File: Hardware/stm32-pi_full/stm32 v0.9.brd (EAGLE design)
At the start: 131.4 x 105.8 mm, 278 parts, among them J1 SOLDERJUMPERNO, Q1 MMBT3906, Q2 MMBT3904, Q3 MMBT3904, U1 ESP32-WROOM-32D, Y1 6MM_3.5MM_CRYSTAL

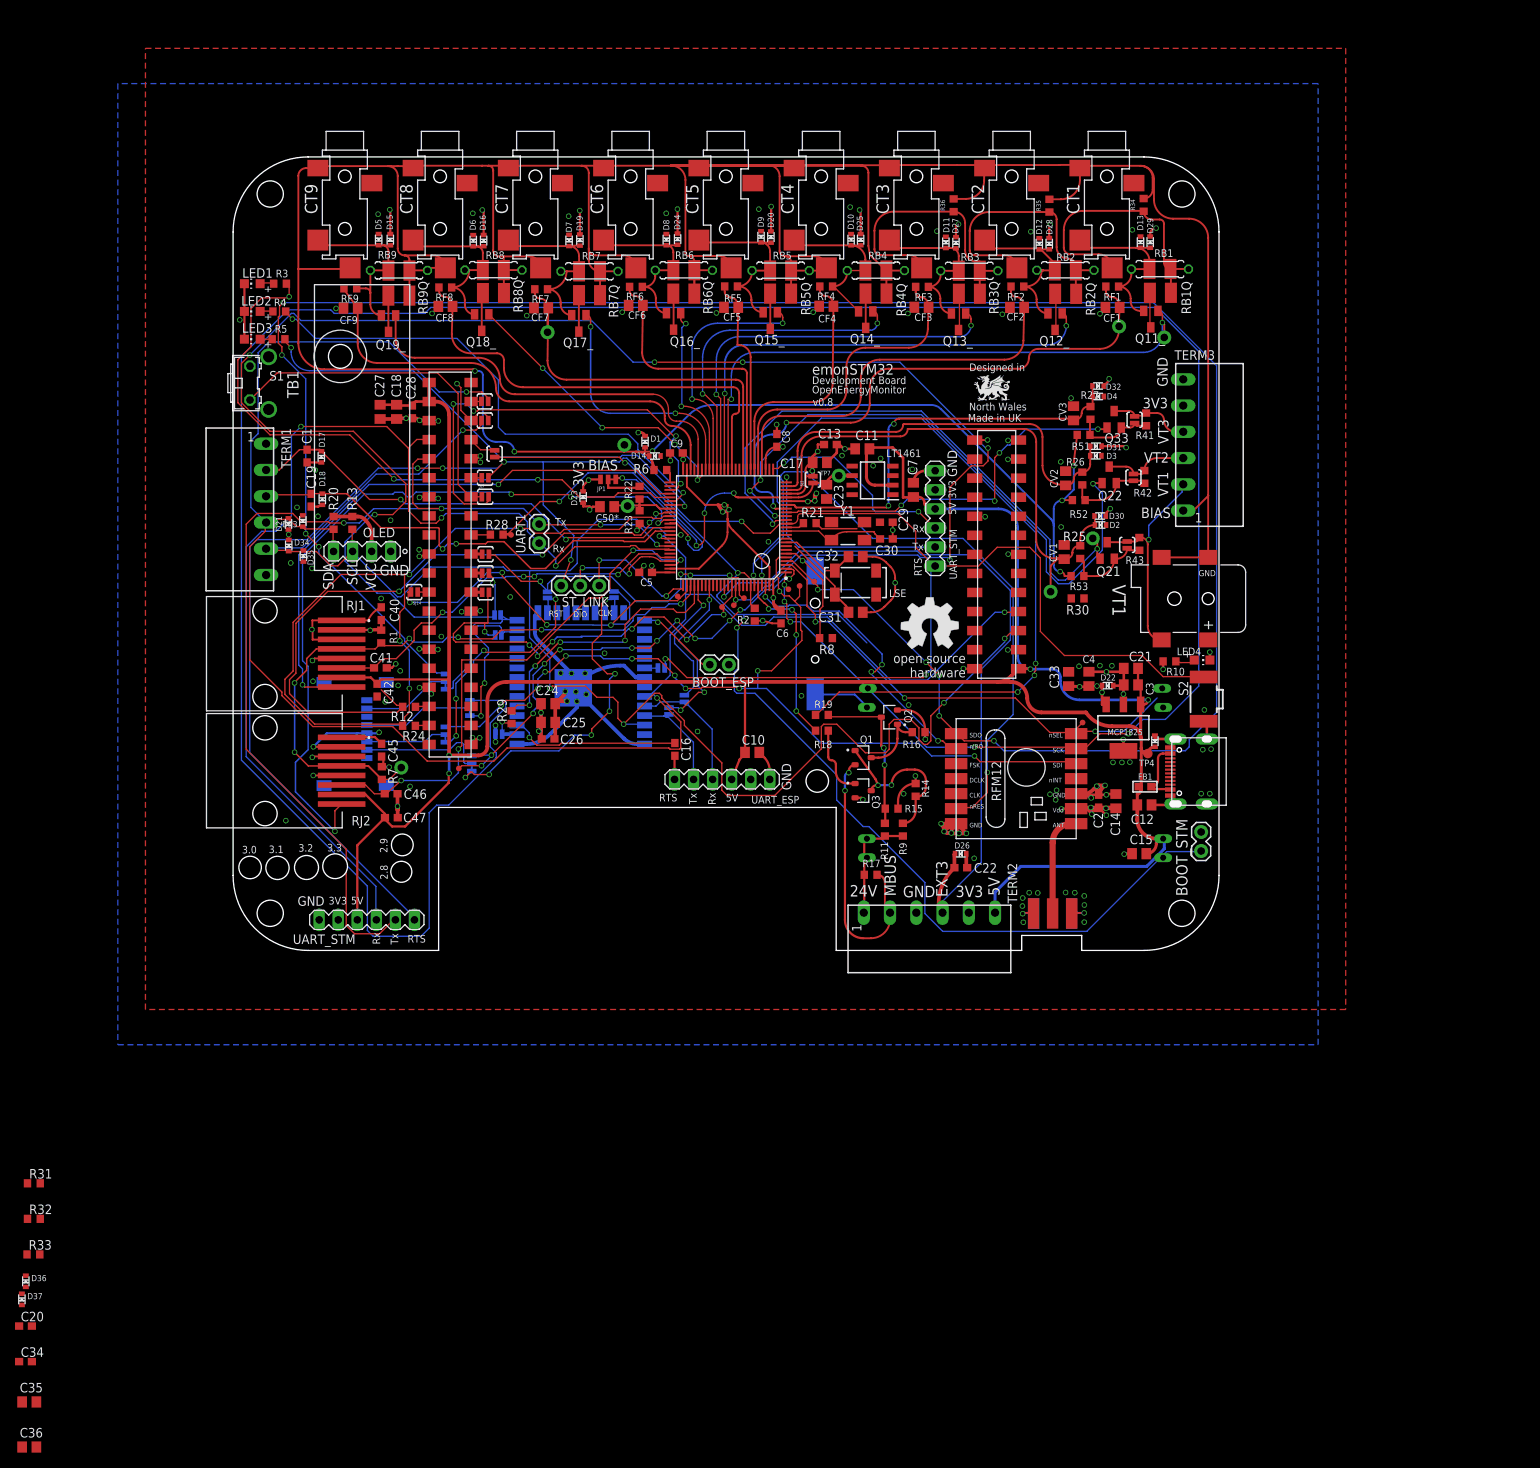
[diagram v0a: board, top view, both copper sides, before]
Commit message: v0.9 backup
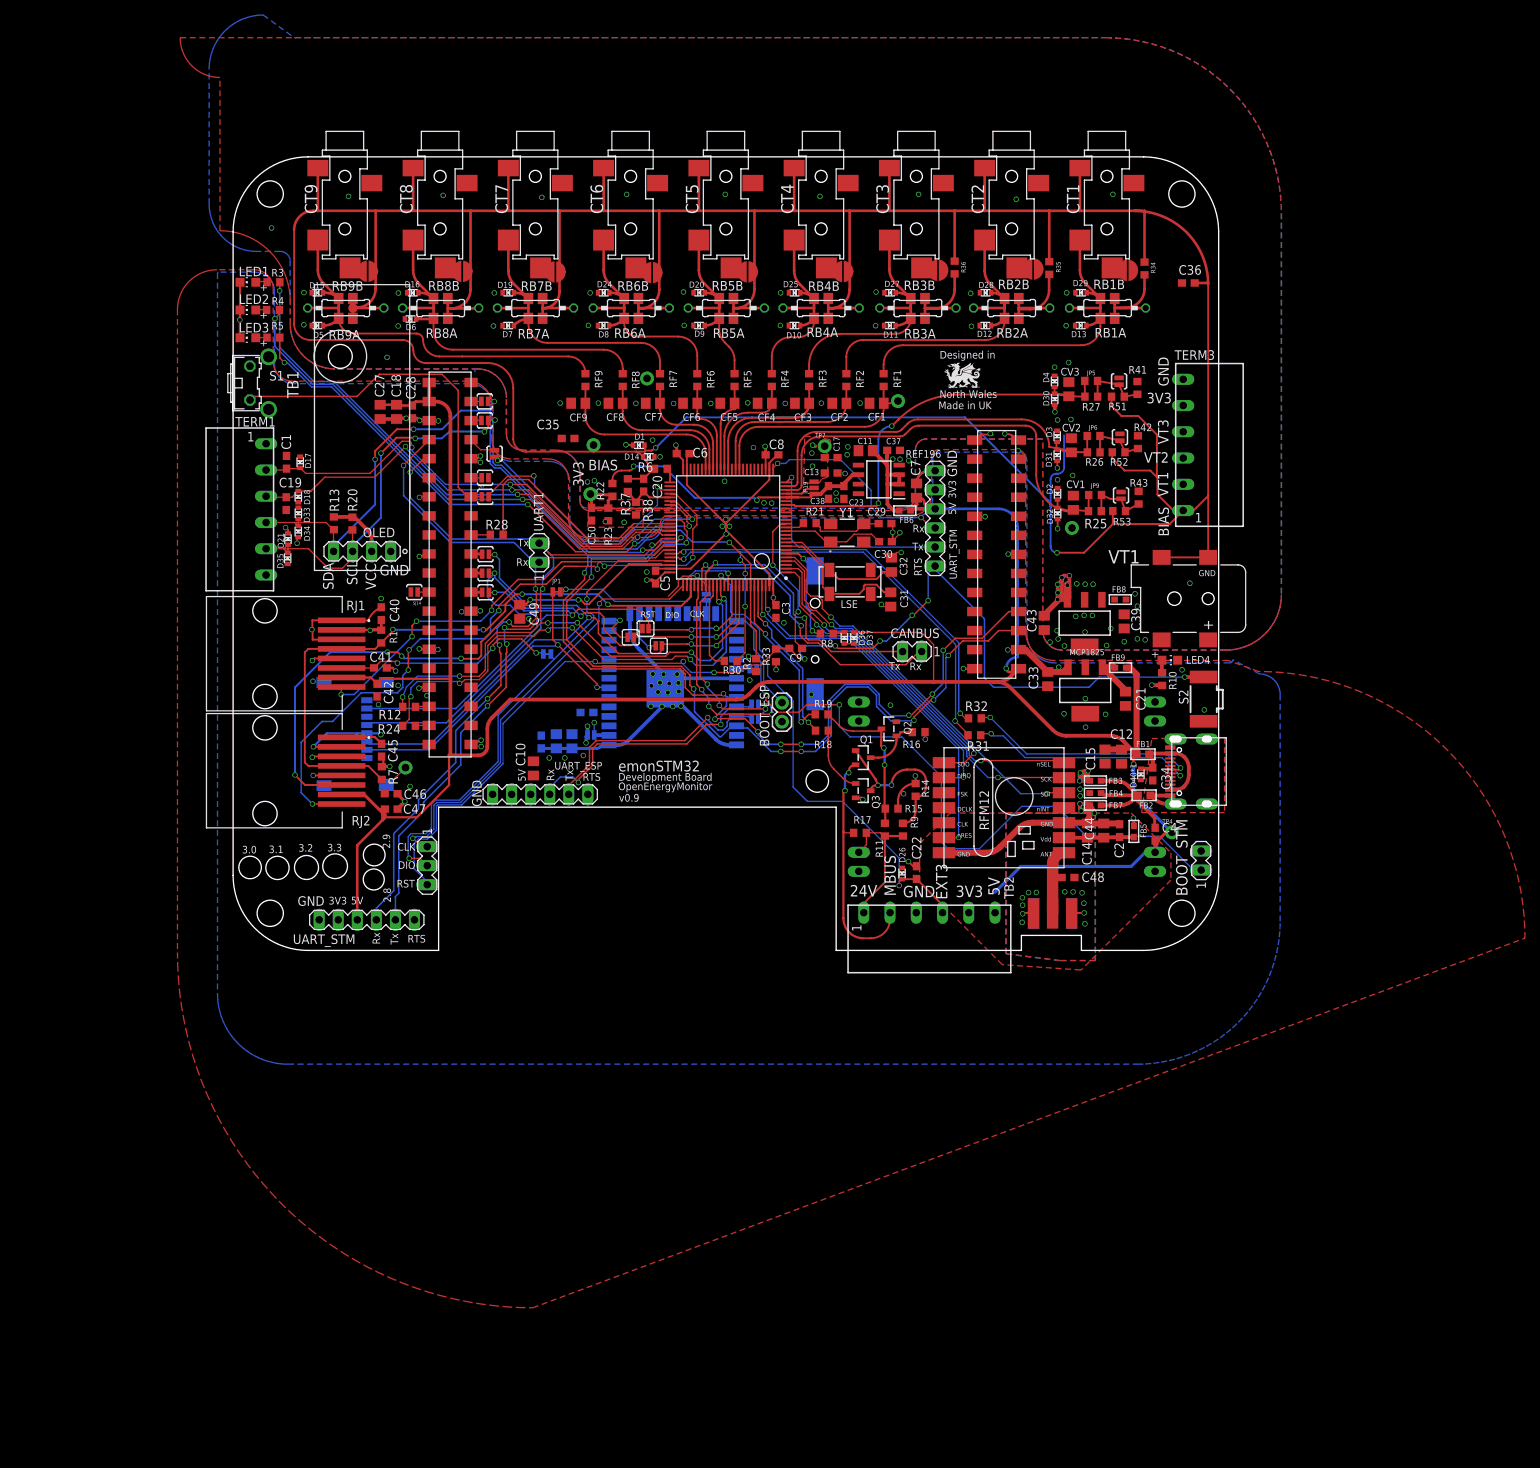
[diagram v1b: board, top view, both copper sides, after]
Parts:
- removed C50*: 2.2uF, rcl:C0805
- removed D22, D23: ESD5Z3.3T1G, microbuilder:SOD-523
- removed GOLD_ORB_SM1: OSHWLOGOLOGO8MM, oshw:OSHW_8MM
- removed JP2, JP3, JP7, JP8: JUMPER-SMT_3_1-NC_TRACE_SILK, SparkFun-Jumpers:SMT-JUMPER_3_1-NC_TRACE_SILK
- removed Q11_, Q12_, Q13_, Q14_, Q15_, Q16_, Q17_, Q18_, Q19_, Q21, Q22, Q33: (no value), adafruit:SOT23
- removed R29: 10K, rcl:R0603
- removed RB1: 22r 0.3W 1%, rcl:R1210
- removed RB1Q, RB2, RB2Q, RB3, RB3Q, RB4, RB4Q, RB5, RB5Q, RB6, RB6Q, RB7, RB7Q, RB8, RB8Q: 22r, rcl:R1210
- removed RB9: 100R 0.1%, rcl:R1210
- removed RB9Q: 22R 0.1%, rcl:R1210
- removed SJ2: SOLDERJUMPERNO, SparkFun:SJ_2S-NO
- removed ST_LINK: 455-1750-1-ND, SparkFun-Connectors:1X03
- removed TP1, TP11, TP12, TP13, TP14, TP15, TP16, TP2, TP21, TP3: TEST-POINT3, SparkFun-Connectors:PAD.03X.03
- removed TP17, TP6: TEST-POINTPOGO_PTH, SparkFun-Connectors:1X01_NO_SILK
- added C37, C38, C48: 100nF, resistor:C0603
- added C39, C43, C44: 22uF, rcl:C0805
- added C49: 10pF, rcl:C0805
- added C50: (no value), rcl:C0603
- added CANBUS: TX/RX, con-lstb-db:MA02-1
- added FB2: (no value), microbuilder:0603
- added FB3, FB4, FB5, FB6, FB7, FB8, FB9: (no value), microbuilder:_0603
- added JP10, JP11, JP12, JP13, JP14, JP15, JP16, JP17, JP18: JUMPER-SMT_2_NO_NO-SILK_ROUND, SparkFun-Jumpers:SMT-JUMPER_2_NO_NO-SILK_ROUND
- added JP19: JUMPER-SMT_3_NO_NO-SILK, SparkFun-Jumpers:SMT-JUMPER_3_NO_NO-SILK
- added JP4: JUMPER-SMT_2_NC_TRACE_NO-SILK, SparkFun-Jumpers:SMT-JUMPER_2_NC_TRACE_NO-SILK
- added JP5, JP6, JP9: 0R, rcl:R0603
- added MCP1825(ANALOG): MCP1825SOT-223-3, SteelCaveRobotics-Power:SOT-223
- added R37: 0R, resistor:R0603
- added R38: 1k, resistor:R0603
- added RB1A, RB1B: 22r 0.3W 1%, rcl:R0805
- added RB2A, RB2B, RB3A, RB3B, RB4A, RB4B, RB5A, RB5B, RB6A, RB6B, RB7A, RB7B, RB8A, RB8B: 22r, rcl:R0805
- added RB9A, RB9B: 100R 0.1%, rcl:R0805
- added SV3: (no value), con-lstb-db:MA03-1
- BOOT_STM, UART1: device SparkFun:1X02 -> con-lstb-db:MA02-1
- C11, C14, C18: value 2.2uF -> 22uF
- C12, C21, C33: value 47uF -> 22uF
- C13, C20: value 100nF -> 2.2uF
- C17, C3, C4: value 2.2uF -> 100nF; device rcl:C0805 -> resistor:C0603
- C23: value 2.2uF -> 1uf; device rcl:C0805 -> rcl:C0603
- C34: device rcl:C0603 -> resistor:C0603
- C35, C36: value 2.2uF -> 1uF; device rcl:C0805 -> rcl:C0603
- C9: value 100nF -> 1uF; device resistor:C0603 -> rcl:C0603
- CT1, CT2, CT3, CT4, CT5, CT6, CT7, CT8, CT9: device IotaWatt_parts:STEREO_SMT -> sj-3523-smt:SJ-352X-SMT
- JP1: value JUMPER-SMT_3_1-NC_TRACE_NO-SILK -> JUMPER-SMT_2_NC_TRACE_NO-SILK; device SparkFun-Jumpers:SMT-JUMPER_3_1-NC_TRACE_NO-SILK -> SparkFun-Jumpers:SMT-JUMPER_2_NC_TRACE_NO-SILK
- Q1: value MMBT3906 -> (none); device Transistor:SOT23 -> microbuilder:SOT23-R
- Q2, Q3: value MMBT3904 -> (none); device Transistor:SOT23 -> microbuilder:SOT23-R
- R25, R26, R27: value 10k -> 9k1
- R30: value 0R -> 1k5; device resistor:R0603 -> rcl:R0603
- R31, R32: value 0R -> 20R; device resistor:R0603 -> rcl:R0603
- R33: value 0R -> 10k
- R41, R42, R43: value 120k -> 100k
- RB1_, RB2_, RB3_, RB4_, RB5_, RB6_, RB7_, RB8_, RB9_: device rcl:0207/7 -> rcl:0207/10
- TP4: value TPB1,27 -> TEST-POINTPOGO_PTH; device testpad:B1,27 -> SparkFun-Connectors:1X01_NO_SILK
- moved C36 219.0 mm to (127.4, 89.0), turned to 180 degrees
- moved C34 169.5 mm to (122.6, 23.5), turned to 270 degrees
- moved C35 147.2 mm to (44.7, 68.3), turned to 180 degrees
- moved R32 142.1 mm to (98.9, 30.9), turned to 180 degrees
- moved D37 140.7 mm to (81.5, 41.7)
- moved D36 139.8 mm to (82.8, 41.7), turned to 180 degrees
- moved C20 139.1 mm to (54.7, 62.0), turned to 270 degrees
- moved R31 138.9 mm to (98.8, 28.7), turned to 180 degrees
- moved R33 127.2 mm to (72.4, 39.3), turned to 90 degrees
- moved C3 48.3 mm to (72.4, 45.2), turned to 270 degrees
- moved R30 47.0 mm to (66.3, 38.6), turned to 180 degrees
- moved CF1 33.9 mm to (85.8, 72.9)
- moved RF9 33.7 mm to (47.0, 76.0), turned to 270 degrees
- moved RF1 32.9 mm to (86.7, 76.0), turned to 270 degrees
- moved CF9 32.9 mm to (46.0, 72.9)
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- renumbered TERM2 to TB2
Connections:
- net BIAS* renamed BIAS_
- net BOOT0 renamed BOOT_STM
- net LED2_YELLOW renamed LED2
- net LED3_RED renamed LED3
- removed net AC1_MOS: Q21.2, R25.1, R30.2, R43.1, R53.1, SJ37.1
- removed net AC2_MOS: Q22.2, R26.1, R31.2, R42.1, R52.1, SJ36.1
- removed net AC3_MOS: Q33.2, R27.1, R32.2, R41.2, R51.1, SJ35.1
- removed net ESP_PWR: R29.2, STM32F303VE.79
- removed net LED1_GREEN: R3.2, STM32F303VE.55
- removed net MOS1: Q11_.1, STM32F303VE.38, TP17.1
- removed net MOS2: Q12_.1, STM32F303VE.39
- removed net MOS3: Q13_.1, STM32F303VE.40
- removed net MOS4: Q14_.1, STM32F303VE.41
- removed net MOS5: Q15_.1, STM32F303VE.42
- removed net MOS6: Q16_.1, STM32F303VE.43
- removed net MOS7: Q17_.1, STM32F303VE.44
- removed net MOS8: Q18_.1, STM32F303VE.45
- removed net MOS9: Q19_.1, STM32F303VE.46
- removed net N$12: JP1.2, R22.2
- removed net N$37: Q14_.3, RB4Q.2
- removed net N$38: CT6.P$2, D24.A, D8.K, Q16_.2, RB6.1, RB6_.1, RF6.1
- removed net N$39: CT5.P$2, D20.A, D9.K, Q15_.2, RB5.1, RB5_.1, RF5.1
- removed net N$40: CT4.P$2, D10.K, D25.A, Q14_.2, RB4.1, RB4_.1, RF4.1
- removed net N$45: Q19_.3, RB9Q.2
- removed net N$46: Q18_.3, RB8Q.2
- removed net N$47: Q15_.3, RB5Q.2
- removed net N$48: Q16_.3, RB6Q.2
- removed net N$49: Q17_.3, RB7Q.2
- removed net N$7: FB1.1, USB-C.A4/B9, USB-C.B4/A9
- removed net SD_CLK: JP8.2, U$7.PIN5
- removed net SD_CS_: JP2.2, U$7.PIN2
- removed net SD_MISO: JP7.2, U$7.PIN7
- removed net SD_MOSI: JP3.2, U$7.PIN3
- removed net SPI4_CS_SDCARD_MASTER: JP2.1, STM32F303VE.2, TP13.P$1
- removed net VMOS1: Q21.1, STM32F303VE.15, TP6.1
- removed net VMOS2: Q22.1, STM32F303VE.16
- removed net VMOS3: Q33.1, STM32F303VE.17
- new net +3V3ANA: C43.1, D1.K, D15.K, D16.K, D19.K, D20.K, D24.K, D25.K, D27.K, D28.K, D29.K, D30.K, D31.K, D32.K, JP19.1, MCP1825(ANALOG).3, TERM3.P$5, TP7.1
- new net +5V_A: C39.1, FB8.1, MCP1825(ANALOG).1
- new net +5V_D: C21.1, FB9.1, MCP1825.1
- new net +5V_REF: C11.1, C37.1, FB6.1, PS1.2, PS1.3
- new net +5V_USB: C34.1, D40*1.K, FB1.1, USB-C.A4/B9, USB-C.B4/A9
- new net AC1_: JP9.2, R25.1, R43.1, R53.1, SJ37.1
- new net AC2_: JP6.2, R26.1, R42.1, R52.1, SJ36.1
- new net AC3_: JP5.2, R27.1, R41.2, R51.1, SJ35.1
- new net AGND: C11.2, C13.2, C17.2, C23.2, C35.2, C36.2, C37.2, C38.2, C39.2, C43.2, C50.1, CF1.1, CF2.1, CF3.1, CF4.1, CF5.1, CF6.1, CF7.1, CF8.1, CF9.1, CV1.2, CV2.2, CV3.2, D10.A, D11.A, D12.A, D13.A, D14.A, D2.A, D3.A, D4.A, D5.A, D6.A, D7.A, D8.A, D9.A, EXPANSION.1, EXPANSION.2, FB3.2, MCP1825(ANALOG).2, MCP1825(ANALOG).4, PS1.4, R23.1, R38.2, STM32F303VE.20, TERM3.P$6
- new net CAN_RX: CANBUS.1, STM32F303VE.81
- new net CAN_TX: CANBUS.2, STM32F303VE.82
- new net CT_IN4: CT4.P$2, D10.K, D25.A, RB4A.1, RB4B.1, RB4_.1, RF4.1
- new net CT_IN5: CT5.P$2, D20.A, D9.K, RB5A.1, RB5B.1, RB5_.1, RF5.1
- new net CT_IN6: CT6.P$2, D24.A, D8.K, RB6A.1, RB6B.1, RB6_.1, RF6.1
- new net CT_IN7: CT7.P$2, D19.A, D7.K, RB7A.1, RB7B.1, RB7_.1, RF7.1
- new net CT_IN8: CT8.P$2, D16.A, D6.K, RB8A.1, RB8B.1, RB8_.1, RF8.1
- new net CT_IN9: CT9.P$2, D15.A, D5.K, RB9A.1, RB9B.1, RB9_.1, RF9.1
- new net DGND: BOOT_ESP.1, C1.2, C10.2, C18.2, C19.2, C21.2, C22.2, C24.2, C25.2, C26.2, C27.2, C28.2, C29.2, C3.2, C30.2, C31.2, C32.2, C33.2, C40.2, C41.2, C42.2, C45.2, C46.2, C47.2, C49.2, C5.2, C6.2, C7.2, C8.2, D17.A, D18.A, D26.A, D33.A, D35.A, EXPANSION.14, EXPANSION.25, EXPANSION.9, FB4.2, G1.-, LED1.C, LED2.C, LED3.C, LED4.C, MCP1825.2, MCP1825.4, OLED.4, PCB2.P$46, PCB2.P$49, PCB2.P$54, PCB2.P$60, PCB2.P$65, PCB2.P$70, PCB2.P$74, PCB2.P$79, Q2.2, Q3.2, R14.1, R15.1, R16.1, R2.2, RJ1.1, RJ1.3, RJ1.5, RJ2.1, RJ2.3, RJ2.5, S2.1, STM32F303VE.27, STM32F303VE.49, STM32F303VE.74, STM32F303VE.99, SV1.1, SV2.1, TB2.P$3, TERM1.P$6, U$2.P$1, U$2.P$2, U$7.P$1, U$7.P$2, U$7.P$3, U$7.P$4, U$7.PIN6, U1.1, U1.15, U1.31, U1.38, U1.39, UART_STM.1
- new net GND_USB: C34.2, D40*1.A, FB2.1, USB-C.A1/B12, USB-C.B1/A12, USB-C.GND1, USB-C.GND2, USB-C.GND3, USB-C.GND4
- new net LED1: R3.2, STM32F303VE.65
- new net N$13: CT3.P$4, JP14.2
- new net N$22: CT8.P$4, JP17.2
- new net NRST_STM_: C9.2, STM32F303VE.14
- new net OPAMP_INVERT-: C20.2, R37.2, R38.1, STM32F303VE.55
- new net RGND: C14.2, C2.2, C44.2, C48.2, FB7.2, J$1.GND@0, J$1.GND@1, J$1.GND@2, J$1.GND@3, RFM69HCW.10, RFM69HCW.7
- new net SD_CARD_STM: JP1.2, STM32F303VE.88
- new net SD_CS: JP1.1, U$7.PIN2, U1.7
- new net USB_DM: R32.2, STM32F303VE.70
- new net USB_DM_: R32.1, USB-C.A7
- new net USB_DP: R30.1, R31.2, STM32F303VE.71
- new net USB_DP_: R31.1, USB-C.A6
- new net USB_RST: R30.2, STM32F303VE.84
- new net VDD: C14.1, C2.1, C44.1, FB5.1, RFM69HCW.9
- new net VDDA: C13.1, C17.1, JP19.2, STM32F303VE.22
- net +3V3: now also C3.1, C5.1, C6.1, C8.1, FB5.2, R13.2, R20.2, R33.1, S1.1; no longer C13.1, C14.1, C17.1, C2.1, C4.2, C5.2, C6.2, C8.2, C9.2, D1.K, D15.K, D16.K, D19.K, D20.K, D22.K, D23.K, D24.K, D25.K, D27.K, D28.K, D29.K, D30.K, D31.K, D32.K, JP1.1, R13.1, R20.1, RFM69HCW.9, SJ2.2, STM32F303VE.22, TERM3.P$5
- net +5V: now also C12.1, C15.1, C4.1, FB6.2, FB8.2, FB9.2, TP4.1; no longer C11.1, C12.2, C15.2, C21.1, C3.1, D40*1.K, MCP1825.1, PS1.2, TP4.TP
- net AC1: no longer Q21.3
- net AC2: no longer Q22.3
- net AC3: no longer Q33.3
- net ANT: now also C48.1
- net BIAS: now also C20.1, JP11.1, JP13.1, JP15.1, JP16.1, JP17.1, JP18.1, R37.1, RB4A.2, RB4B.2, RB5A.2, RB5B.2, RB6A.2, RB6B.2, RB7A.2, RB7B.2, RB8A.2, RB8B.2, RB9A.2, RB9B.2; no longer CT4.P$4, CT5.P$4, CT6.P$4, CT7.P$4, CT8.P$4, CT9.P$4, RB4.2, RB4Q.1, RB5.2, RB5Q.1, RB6.2, RB6Q.1, RB7.2, RB7Q.1, RB8.2, RB8Q.1, RB9.2, RB9Q.1
- net BIAS_IN: now also C50.2; no longer C50*.2
- net CT1: now also STM32F303VE.35; no longer STM32F303VE.18
- net CT2: now also STM32F303VE.36; no longer STM32F303VE.29
- net CT3: now also STM32F303VE.38; no longer STM32F303VE.30
- net CT4: now also STM32F303VE.39; no longer STM32F303VE.31
- net CT5: now also STM32F303VE.40; no longer STM32F303VE.32
- net CT6: now also STM32F303VE.41; no longer STM32F303VE.33
- net CT7: now also STM32F303VE.42; no longer STM32F303VE.34
- net CT8: now also STM32F303VE.43; no longer STM32F303VE.37
- net CT9: now also STM32F303VE.44; no longer STM32F303VE.48
- net CT_IN1: now also RB1A.1, RB1B.1; no longer Q11_.2, RB1.1
- net CT_IN2: now also RB2A.1, RB2B.1; no longer Q12_.2, RB2.1
- net CT_IN3: now also RB3A.1, RB3B.1; no longer Q13_.2, RB3.1
- net ESP_PWR_PRE: no longer R29.1
- net GND: now also C12.2, C15.2, C4.2, FB2.2, FB3.1, FB4.1, FB7.1; no longer BOOT_ESP.1, C1.2, C10.2, C11.2, C12.1, C13.2, C14.2, C15.1, C17.2, C18.2, C19.2, C2.2, C20.2, C21.2, C22.2, C23.2, C24.2, C25.2, C26.2, C27.2, C28.2, C29.2, C3.2, C30.2, C31.2, C32.2, C33.2, C35.2, C36.2, C4.1, C40.2, C41.2, C42.2, C45.2, C46.2, C47.2, C5.1, C50*.1, C6.1, C7.2, C8.1, C9.1, CF1.1, CF2.1, CF3.1, CF4.1, CF5.1, CF6.1, CF7.1, CF8.1, CF9.1, CV1.2, CV2.2, CV3.2, D10.A, D11.A, D12.A, D13.A, D14.A, D17.A, D18.A, D2.A, D22.A, D23.A, D26.A, D3.A, D33.A, D35.A, D4.A, D40*1.A, D5.A, D6.A, D7.A, D8.A, D9.A, EXPANSION.1, EXPANSION.14, EXPANSION.2, EXPANSION.25, EXPANSION.9, G1.-, J$1.GND@0, J$1.GND@1, J$1.GND@2, J$1.GND@3, LED1.C, LED2.C, LED3.C, LED4.C, MCP1825.2, MCP1825.4, OLED.4, PCB2.P$46, PCB2.P$49, PCB2.P$54, PCB2.P$60, PCB2.P$65, PCB2.P$70, PCB2.P$74, PCB2.P$79, PS1.4, Q2.2, Q3.2, R14.1, R15.1, R16.1, R2.2, R23.1, RFM69HCW.10, RFM69HCW.7, RJ1.1, RJ1.3, RJ1.5, RJ2.1, RJ2.3, RJ2.5, S1.1, S2.1, STM32F303VE.20, STM32F303VE.49, STM32F303VE.74, STM32F303VE.99, SV1.1, SV2.1, TB2.P$3, TERM1.P$6, TERM3.P$6, U$2.P$1, U$2.P$2, U$7.P$1, U$7.P$2, U$7.P$3, U$7.P$4, U$7.PIN6, U1.1, U1.15, U1.31, U1.38, U1.39, UART_STM.1, USB-C.A1/B12, USB-C.B1/A12, USB-C.GND1, USB-C.GND2, USB-C.GND3, USB-C.GND4
- net HSPI_CLK: no longer JP8.3
- net HSPI_CS0: no longer JP2.3
- net HSPI_ID/MOSI: no longer JP3.3
- net HSPI_Q/MISO: no longer JP7.3
- net N$1: now also CT1.P$4, JP10.2; no longer R33.2, STM32F303VE.8
- net N$10: now also CT5.P$4, JP13.2; no longer CT7.P$2, D19.A, D7.K, Q17_.2, RB7.1, RB7_.1, RF7.1
- net N$2: now also CT4.P$4, JP11.2; no longer CT9.P$2, D15.A, D5.K, Q19_.2, RB9.1, RB9_.1, RF9.1
- net N$20: now also CT6.P$4, JP15.2; no longer Q11_.3, RB1Q.2
- net N$21: now also CT9.P$4, JP16.2; no longer Q12_.3, RB2Q.2
- net N$23: now also CT7.P$4, JP18.2; no longer Q13_.3, RB3Q.2
- net N$26: now also JP10.1, RB1A.2, RB1B.2; no longer CT1.P$4, RB1.2, RB1Q.1
- net N$27: now also JP12.1, RB2A.2, RB2B.2; no longer CT2.P$4, RB2.2, RB2Q.1
- net N$28: now also JP14.1, RB3A.2, RB3B.2; no longer CT3.P$4, RB3.2, RB3Q.1
- net N$8: now also CT2.P$4, JP12.2; no longer CT8.P$2, D16.A, D6.K, Q18_.2, RB8.1, RB8_.1, RF8.1
- net NRST_STM: now also C9.1, R33.2, SV3.3; no longer C34.1, C34.2, STM32F303VE.14, ST_LINK.3
- net PC14: now also STM32F303VE.8; no longer R33.1
- net PULSE1_RJ45: now also JP4.1; no longer STM32F303VE.71
- net PULSE_2_RJ45: now also C49.1
- net RPI_GPIO16: now also STM32F303VE.85; no longer STM32F303VE.59
- net RPI_GPIO20: now also STM32F303VE.86; no longer STM32F303VE.60
- net RPI_PWR: no longer TP11.P$1
- net SCL: now also R20.1, STM32F303VE.67; no longer R13.2, STM32F303VE.65
- net SDA: now also R13.1; no longer R20.2
- net SPI1_CLK_SLAVE: now also U$7.PIN5; no longer TP1.P$1
- net SPI1_MISO_SLAVE: now also U$7.PIN7; no longer TP2.P$1
- net SPI1_MOSI_SLAVE: now also U$7.PIN3; no longer TP3.P$1
- net SPI1_NSS_SLAVE: no longer TP21.P$1
- net SPI4_CLK_MASTER: no longer JP8.1, TP12.P$1
- net SPI4_CS_RFM69_MASTER: now also STM32F303VE.2; no longer STM32F303VE.3, TP14.P$1
- net SPI4_MISO_MASTER: no longer JP7.1, TP15.P$1
- net SPI4_MOSI_MASTER: no longer JP3.1, TP16.P$1
- net SWCLK: now also SV3.1; no longer ST_LINK.1
- net SWDIO: now also JP4.2, SV3.2; no longer ST_LINK.2
- net VBAT: no longer C20.1
- net VREF+: now also C38.1, JP19.3, R22.2; no longer JP1.3, SJ2.1, TP7.1
- net VSIG1: now also D32.A, JP9.1; no longer D30.A, R30.1
- net VSIG2: now also JP6.1; no longer R31.1
- net VSIG3: now also D30.A, JP5.1; no longer D32.A, R32.1
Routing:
- net SPI4_CLK_MASTER: track 383.8 -> 51.2 mm, vias 5 -> 2
- net GND: track 295.6 -> 21.2 mm, vias 142 -> 0
- net SPI4_MISO_MASTER: track 308.0 -> 42.8 mm, vias 9 -> 2
- net DGND: track 0.00 -> 191.1 mm, vias 0 -> 74
- net SPI1_MISO_SLAVE: track 238.1 -> 84.8 mm, vias 8 -> 4
- net NRST_STM: track 288.0 -> 150.7 mm, vias 7 -> 9
- net +3V3ANA: track 0.00 -> 123.3 mm, vias 0 -> 22
- net USART3_RX: track 111.8 -> 23.0 mm, vias 4 -> 2
- net LED1_GREEN: track 84.3 -> 0.00 mm, vias 3 -> 0
- net VMOS2: track 83.2 -> 0.00 mm, vias 4 -> 0
- net VMOS1: track 79.4 -> 0.00 mm, vias 2 -> 0
- net MOS1: track 78.0 -> 0.00 mm, vias 2 -> 0
- net +3V3: track 143.0 -> 68.5 mm, vias 40 -> 18
- net LED1: track 0.00 -> 72.7 mm, vias 0 -> 2
- net USB_DP: track 0.00 -> 71.7 mm, vias 0 -> 5
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- added copper zone on layer 1, net +3V3ANA
- added copper zone on layer 15, net +3V3ANA
- added copper zone on layer 1, net AGND
- added copper zone on layer 16, net AGND
- added copper zone on layer 2, net AGND
- added copper zone on layer 1, net DGND
- added copper zone on layer 16, net DGND
- added copper zone on layer 2, net DGND
- added copper zone on layer 1, net GND_USB
- added copper zone on layer 1, net RGND
- added copper zone on layer 16, net RGND
- added copper zone on layer 2, net RGND
- removed copper zone on layer 1, net GND
- removed copper zone on layer 16, net GND
- removed copper zone on layer 2, net GND
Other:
- board text added: "131.4 x 105.8 y"
- board text added: "REF196"
- board text added: "v0.9"
- board text removed: "131.445 x 105.791 y"
- board text removed: "LT1461"
- board text removed: "TP4"
- board text removed: "v0.8"

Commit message: v0.9 for checking
update PCB and enclosure
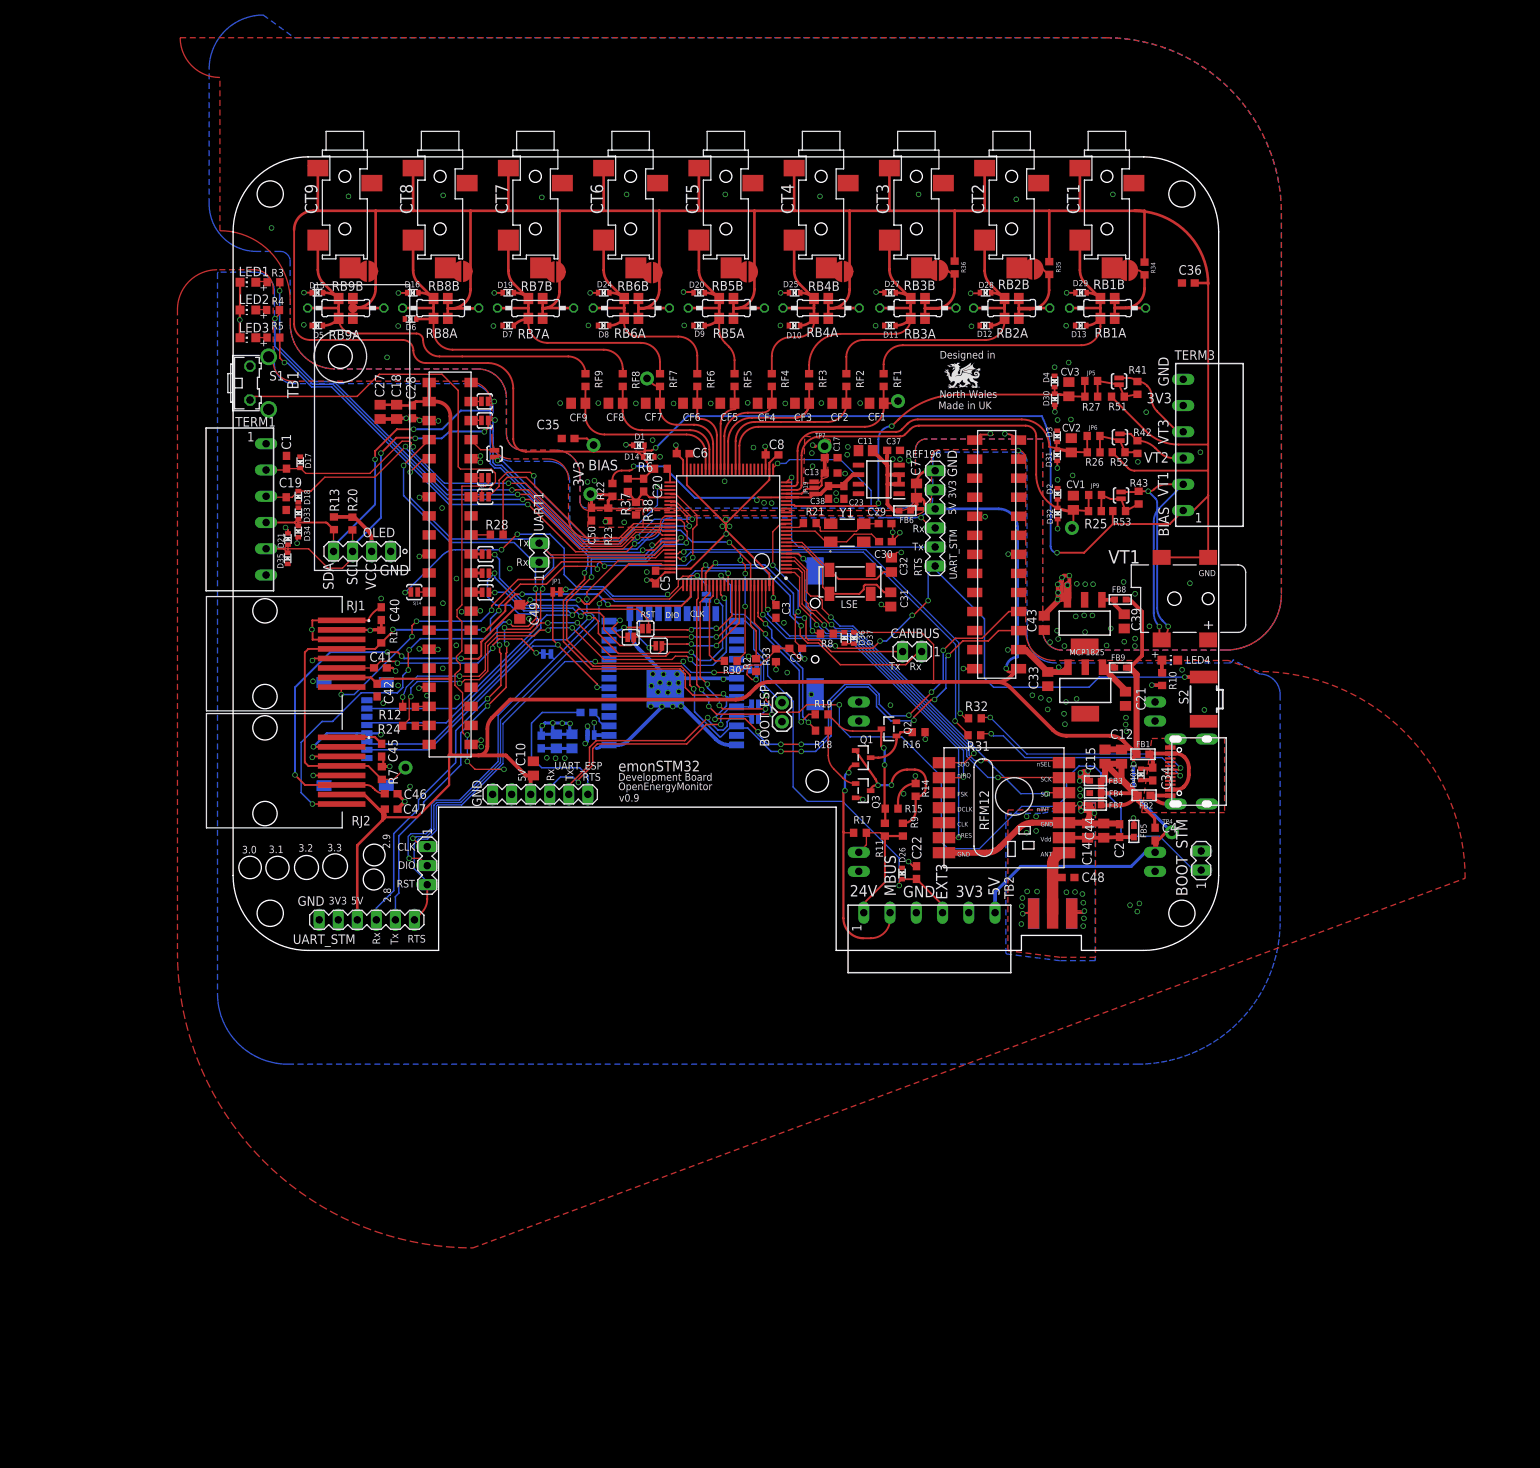
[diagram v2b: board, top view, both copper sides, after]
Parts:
- moved R42 0.66 mm to (120.6, 67.1)
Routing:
- net +3V3ANA: track 123.3 -> 63.8 mm
- net NRST_STM: track 150.7 -> 209.8 mm, vias 9 -> 13
- net AC1: track 0.13 -> 52.0 mm, vias 0 -> 3
- net SPI1_NSS_SLAVE: track 9.82 -> 54.5 mm, vias 1 -> 5
- net +5V: track 335.9 -> 361.7 mm
- net N$14: track 0.00 -> 22.7 mm
- net GND: track 21.2 -> 40.4 mm
- net +3V3: track 68.5 -> 82.2 mm, vias 18 -> 22
- net AC3: track 0.00 -> 12.1 mm
- net AC2: track 0.00 -> 9.40 mm
- net BOOT_STM: track 143.2 -> 152.5 mm
- net +5V_A: track 0.00 -> 6.67 mm
- net PULSE_2_RJ45: track 79.3 -> 85.3 mm
- net VDDA: track 3.85 -> 9.04 mm
- net BUTTON1: track 46.7 -> 51.8 mm
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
